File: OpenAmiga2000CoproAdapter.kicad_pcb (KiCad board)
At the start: 2 copper layers, 188.6 x 114.2 mm, 74 parts, among them CN1 A2000_COPRO_SLOT, P1 CONN_2, P10 CONN_1, P11 CONN_1, P12 CONN_1, P13 CONN_1, P14 CONN_1, P15 CONN_1, P2 CONN_2, P3 CONN_2, P4 CONN_2, P5 CONN_1, P6 CONN_1, P7 CONN_1, P8 CONN_1, P9 CONN_1, P99 OSHW_LOGO, U1 68000D, U10 Spare, U11 74HCT00, U12 74HCT27, U13 74HCT74, U14 74F86, U15 74F74, U16 74HCT04, U17 74HCT112, U18 74F157, U19 74F157, U2 AS6C4008-55PCN, U3 AS6C4008-55PCN, U4 AS6C4008-55PCN, U5 AS6C4008-55PCN, U6 74HCT00, U7 74HCT32, U8 74HCT32, U9 74LS05

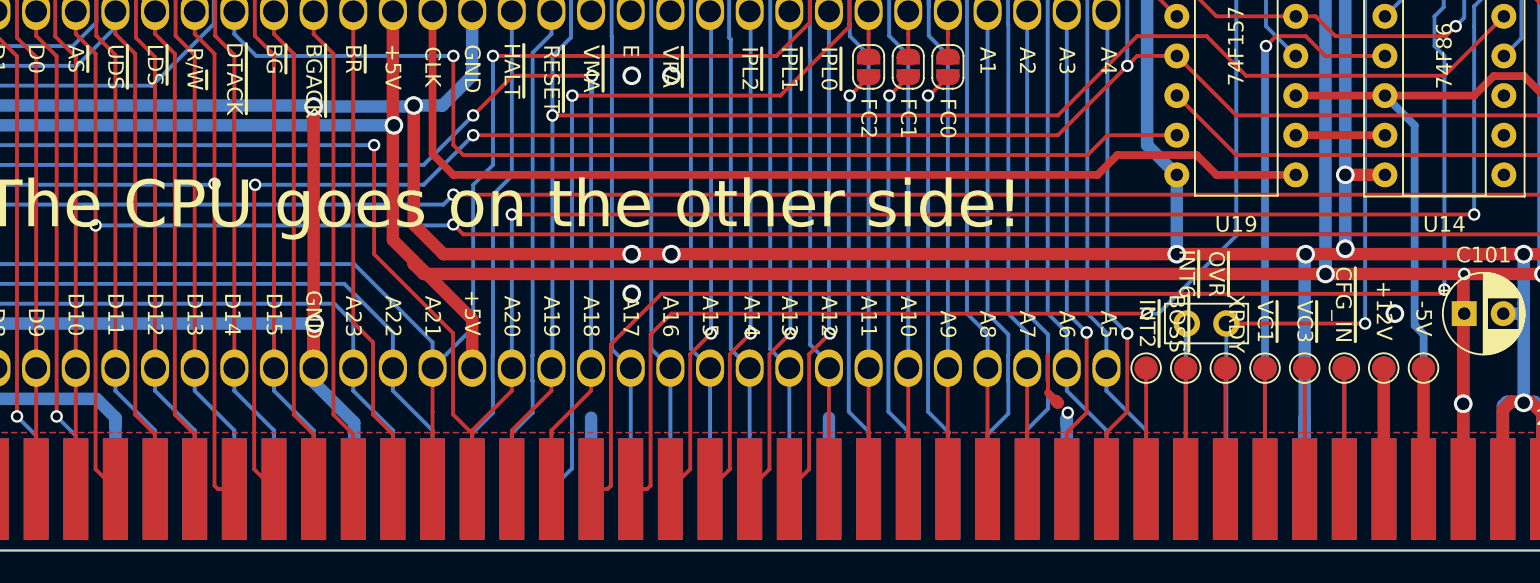
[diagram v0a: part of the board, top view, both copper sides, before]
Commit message: fix connector
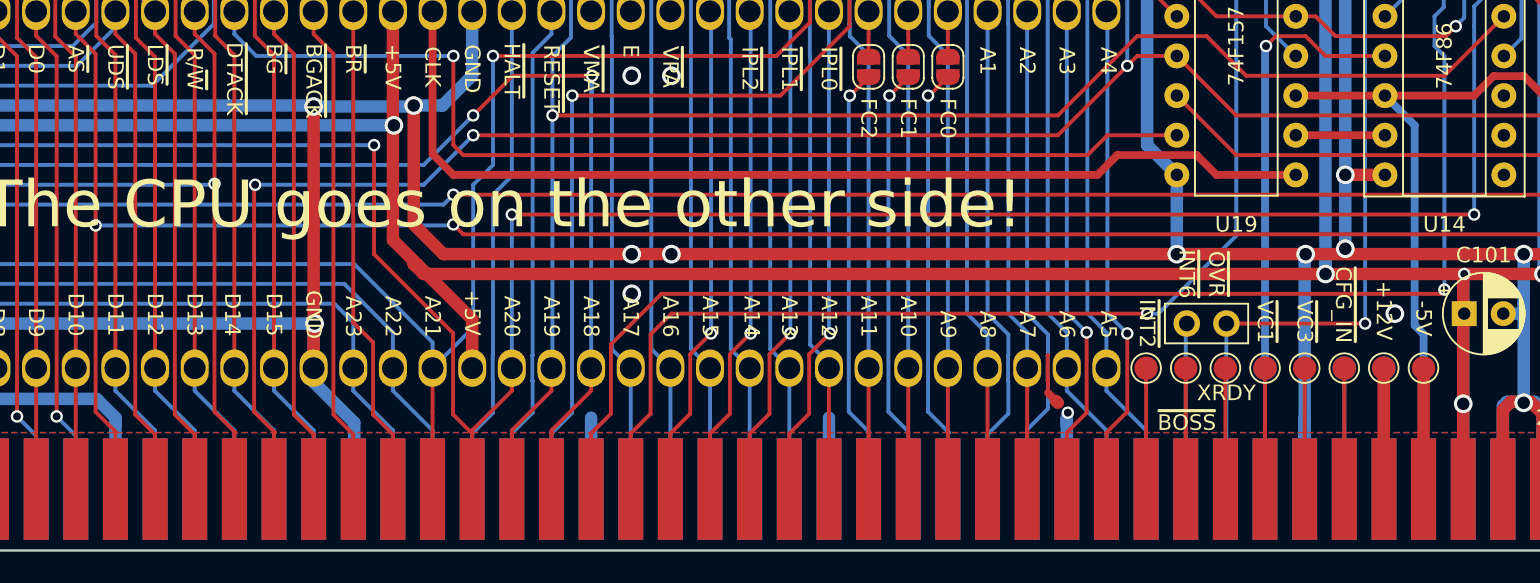
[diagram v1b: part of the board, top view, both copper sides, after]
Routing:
- net /~vpa: track 135.8 -> 135.2 mm
- net /e: track 105.2 -> 104.6 mm
- net /r_~w: track 191.0 -> 190.4 mm
